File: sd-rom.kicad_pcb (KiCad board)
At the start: 2 copper layers, 171.1 x 100 mm, 4 parts, among them J1 JAE50, J2 Conn_01x40, J3 Conn_01x40, J4 SD44

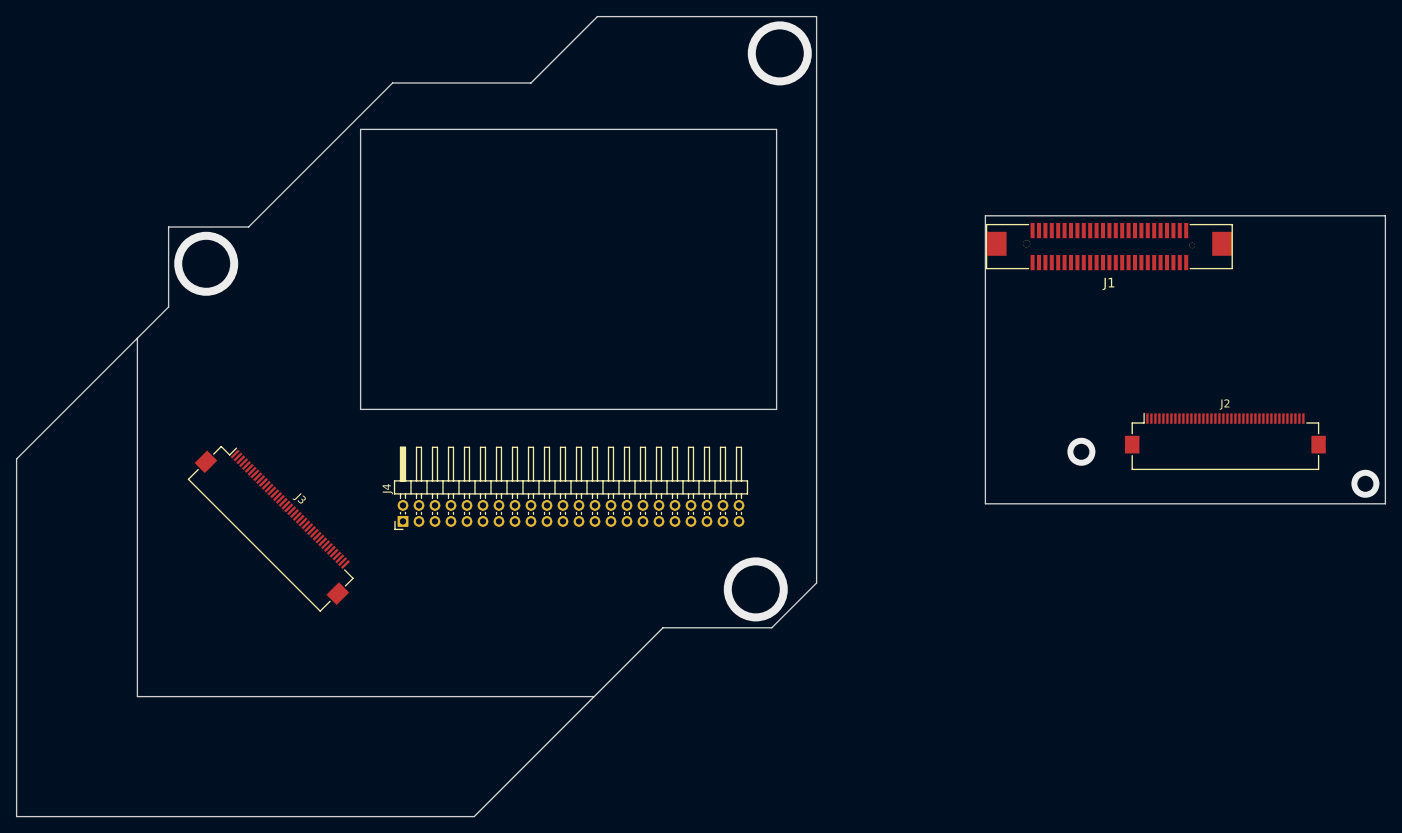
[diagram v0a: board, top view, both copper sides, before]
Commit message: board variant 2
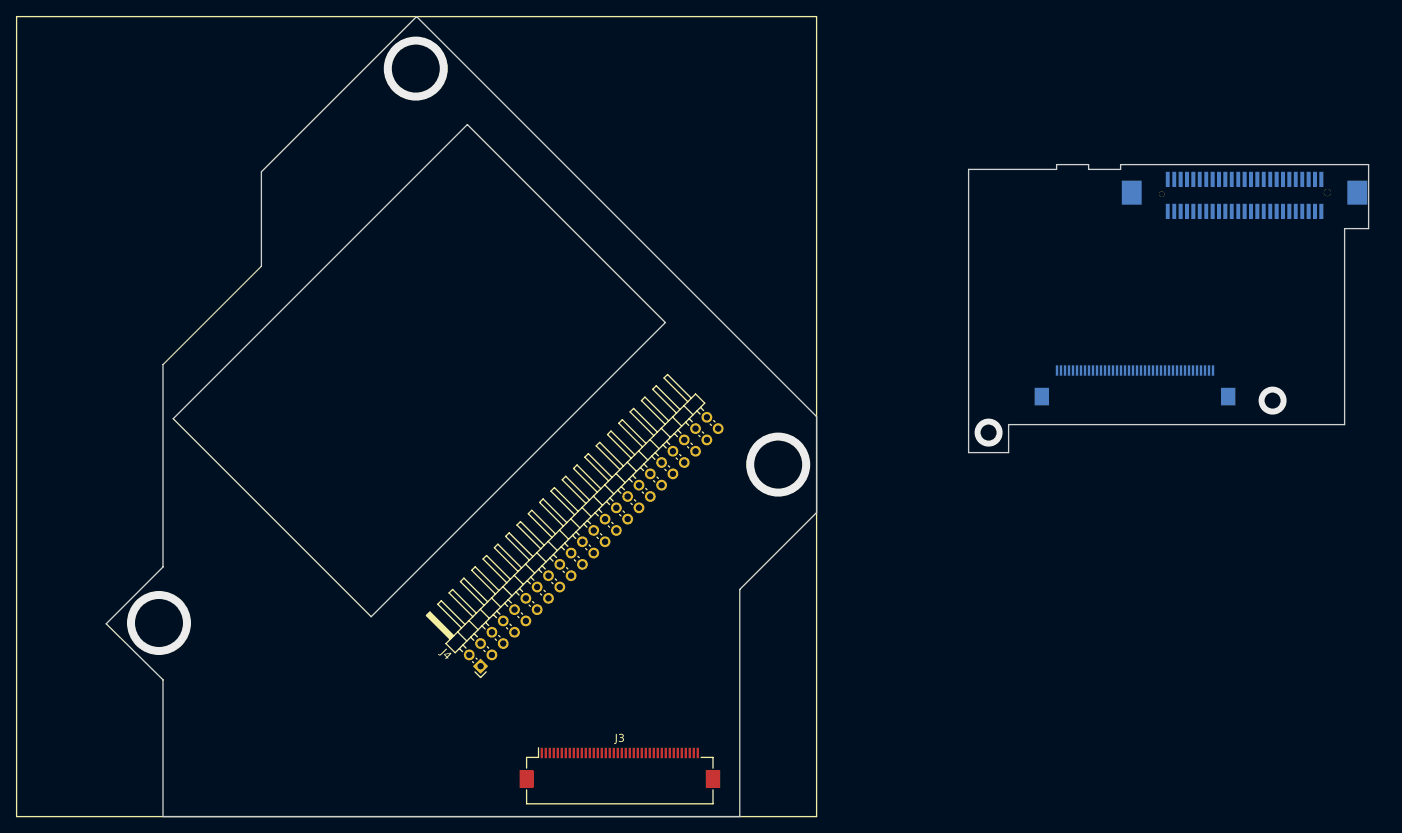
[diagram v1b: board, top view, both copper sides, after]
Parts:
- J1, J2: moved to B.Cu
- moved J3 52.6 mm to (75.4, 93.9), turned to 0 degrees
- moved J4 20.5 mm to (58.0, 81.2), turned to 135 degrees
- moved J2 12.8 mm to (139.8, 46.1), turned to 180 degrees
- moved J1 7.44 mm to (143.2, 19.4), turned to 180 degrees
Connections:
- J1 pad : GNDREF -> (no net)
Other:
- board size 171.1 x 100 mm -> 157.8 x 100 mm
